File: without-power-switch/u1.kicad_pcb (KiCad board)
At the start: 2 copper layers, 18 x 16.5 mm, 12 parts, among them J1 USB_C_Receptacle_USB2.0, J2 Conn_01x06_MountingPin, U1 USBLC6-2P6

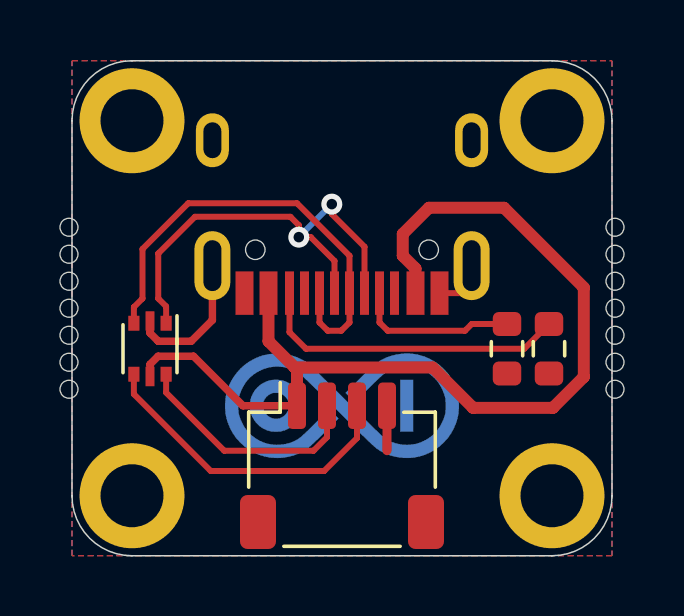
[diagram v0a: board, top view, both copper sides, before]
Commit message: Add rendering files
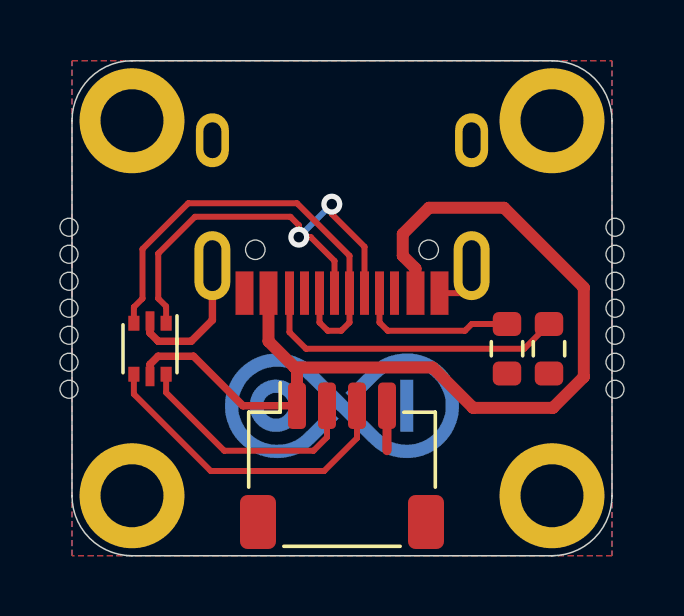
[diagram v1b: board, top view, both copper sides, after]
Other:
- net class Default removed
